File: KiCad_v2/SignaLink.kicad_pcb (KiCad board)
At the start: 2 copper layers, 60 x 45 mm, 68 parts, among them Q1 MMBT3904, SW1 SW_Wake, U1 DM-OLED096-636, U2 ESP32-C3_SUPERMINI_TH, U3 MIC94063YC6-TR, U4 CM4102008, U5 LT8582EDKD-PBF, U6 MCP73871, U7 LM3940IMP-3.3, U8 BNO085, U9 MPU-6050

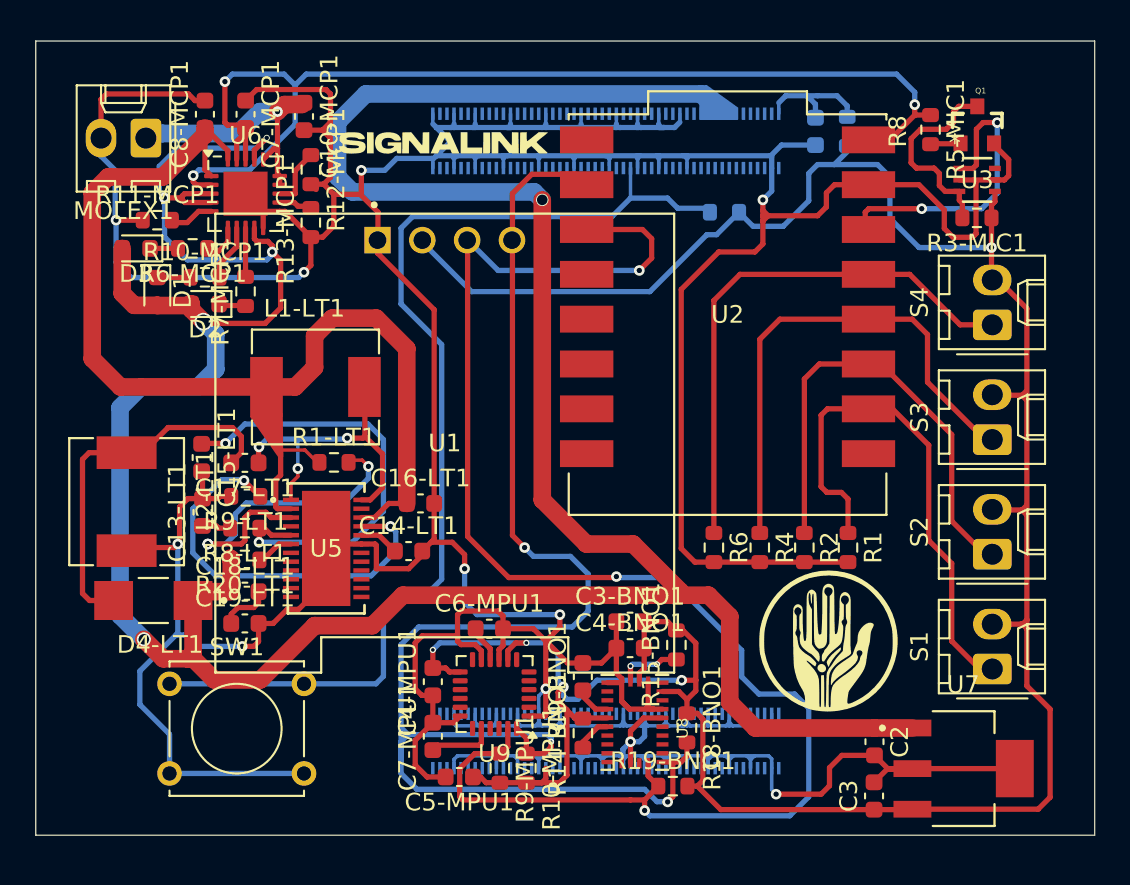
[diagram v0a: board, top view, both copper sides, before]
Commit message: modificaciones en silkscreen
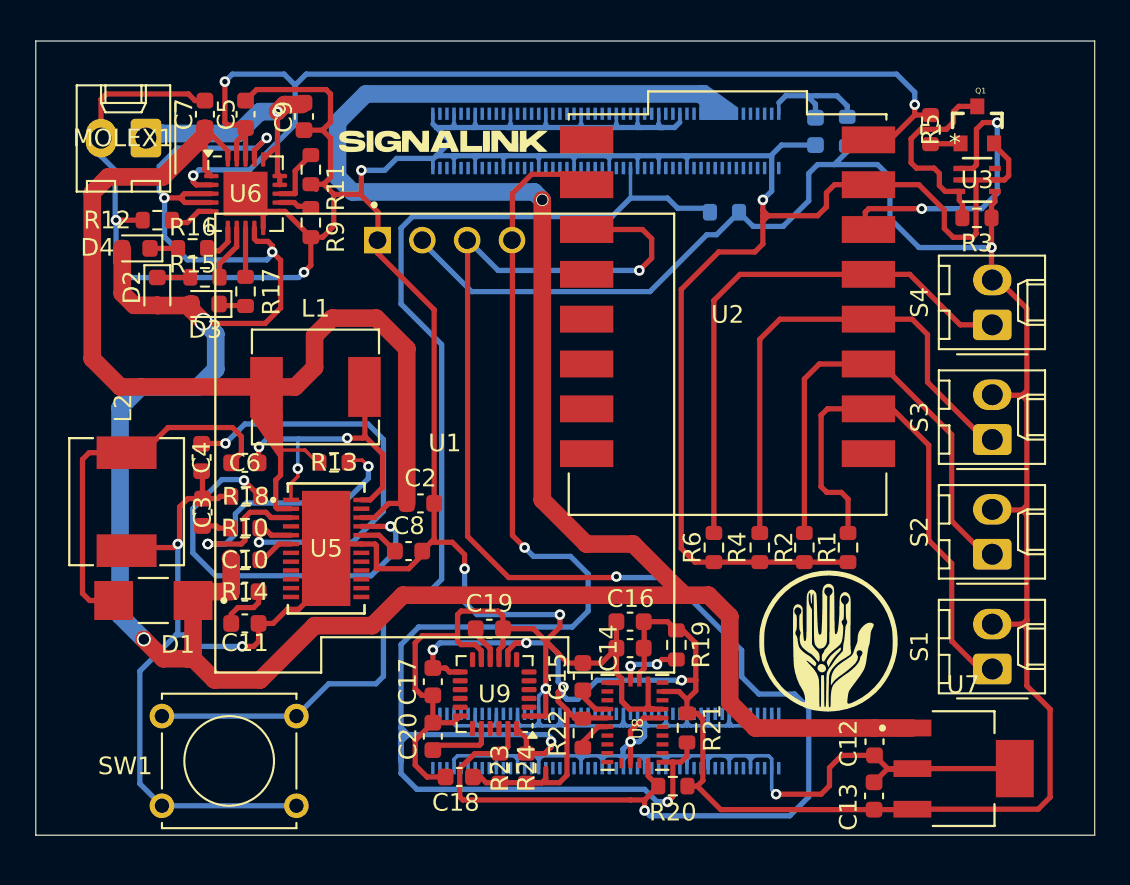
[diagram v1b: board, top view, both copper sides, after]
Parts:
- D2: renamed from D1; value LED-MCP -> LED
- D3: renamed from D2; value LED-MCP -> LED
- D4: renamed from D3; value LED-MCP -> LED
- R5: renamed from R5-MIC1; value 100k -> 4k7
- moved SW1 1.88 mm to (25.9, 85.8)
- moved G*** 0.09 mm to (41.9, 53.6)
- renumbered C18-LT1 to C10, C19-LT1 to C11, C2 to C12, C3 to C13, C4-BNO1 to C14, C9-BNO1 to C15, C3-BNO1 to C16, C4-MPU1 to C17, C5-MPU1 to C18, C6-MPU1 to C19, C16-LT1 to C2, C7-MPU1 to C20, C13-LT1 to C3, C15-LT1 to C4, C7-MCP1 to C5, C17-LT1 to C6, C8-MCP1 to C7, C14-LT1 to C8, C10-MCP1 to C9, D4-LT1 to D1, L1-LT1 to L1, L2-LT1 to L2, R8-LT1 to R10, R12-MCP1 to R11, R11-MCP1 to R12, R1-LT1 to R13, R20-LT1 to R14, R10-MCP1 to R15, R6-MCP1 to R16, R7-MCP1 to R17, R9-LT1 to R18, R15-BNO1 to R19, R19-BNO1 to R20, R18-BNO1 to R21, R14-BNO1 to R22, R9-MPU1 to R23, R10-MPU1 to R24, R3-MIC1 to R3, R13-MCP1 to R9
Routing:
- net GND: track 408.1 -> 409.8 mm
- net Net-(U4A-GPIO2): track 61.0 -> 62.2 mm
